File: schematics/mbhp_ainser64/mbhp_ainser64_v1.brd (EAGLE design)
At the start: 100 x 80 mm, 43 parts, among them IC1 MCP3208, IC10 4051, IC11 4051, IC2 74HC595, IC3 7805, IC4 4051, IC5 4051, IC6 4051, IC7 4051, IC8 4051, IC9 4051

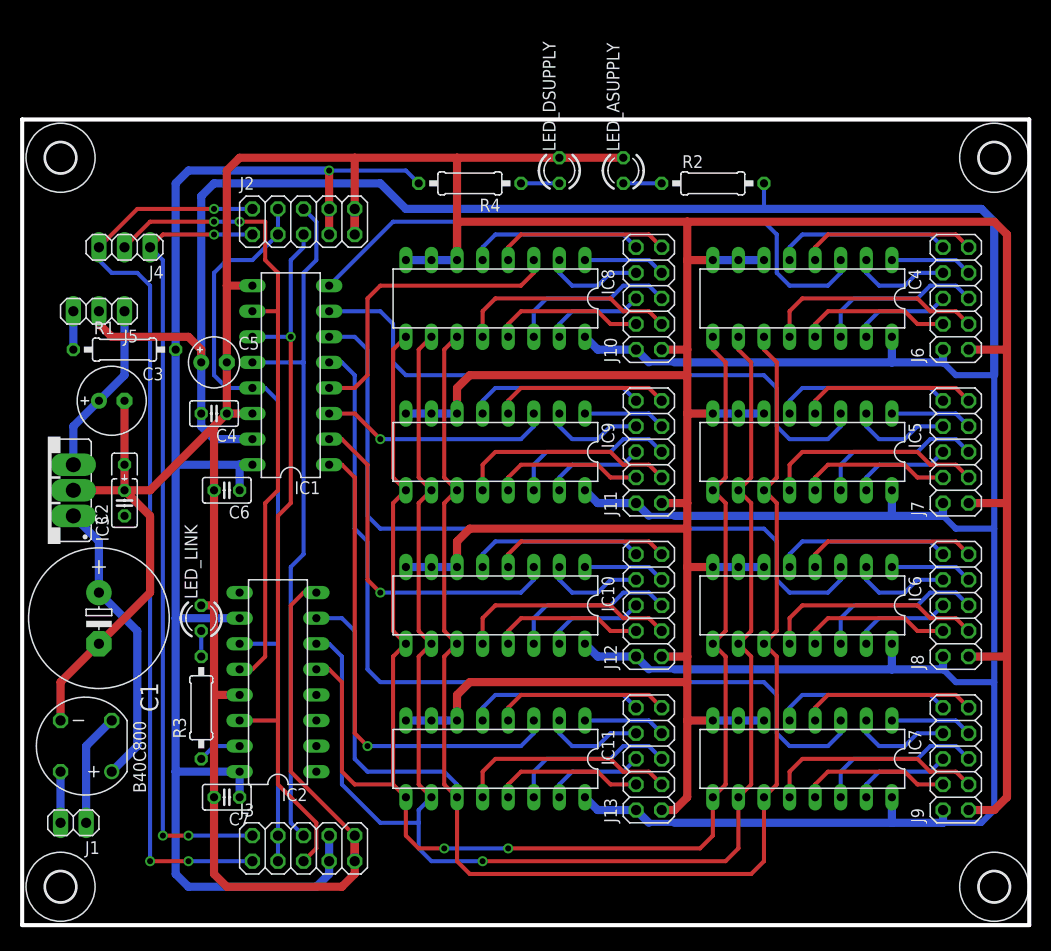
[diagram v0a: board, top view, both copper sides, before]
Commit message: MBHP_AINSER64: layout updates
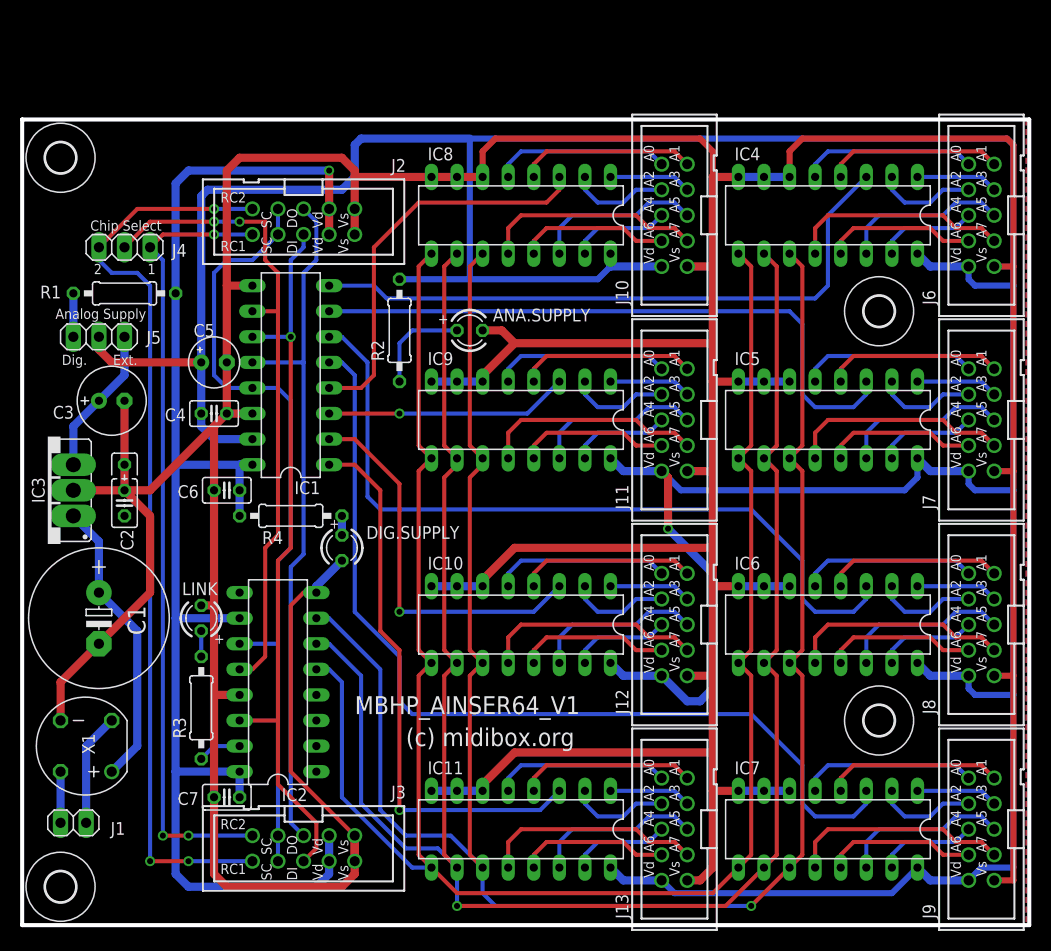
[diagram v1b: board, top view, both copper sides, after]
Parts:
- removed LED_ASUPPLY, LED_DSUPPLY: (no value), led:LED3MM
- added ANA.SUPPLY, DIG.SUPPLY: (no value), led:LED3MM
- J10, J11, J12, J13, J2, J3, J6, J7, J8, J9: device pinhead:2X05 -> con-3m:PAK100/2500-10
- X1: value (none) -> B40C800
- moved R4 37.5 mm to (26.7, 40.6)
- moved R2 34.4 mm to (37.5, 59.1), turned to 90 degrees
- moved E$8 20.1 mm to (85.1, 20.3)
- moved E$7 19.0 mm to (85.1, 61.0)
- moved IC4 8.64 mm to (80.0, 70.5)
- moved J6 8.64 mm to (95.2, 70.5)
- moved IC8 8.64 mm to (49.5, 70.5)
- moved J10 8.64 mm to (64.8, 70.5)
- moved IC7 7.43 mm to (80.0, 9.53)
- moved J9 7.43 mm to (95.2, 9.53)
- moved IC11 7.43 mm to (49.5, 9.53)
- moved J13 7.43 mm to (64.8, 9.53)
- moved R1 5.59 mm to (10.2, 62.7)
- moved IC5 4.07 mm to (80.0, 50.2)
- moved J7 4.07 mm to (95.2, 50.2)
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- renumbered B40C800 to X1, LED_LINK to LINK
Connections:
- net S$70 renamed S$80
- removed net S$10: IC5.5, J7.10
- removed net S$20: IC6.4, J8.9
- removed net S$30: IC7.2, J9.8
- removed net S$40: IC8.1, J10.7
- removed net S$50: IC9.15, J11.6
- removed net S$60: IC10.14, J12.5
- new net S$74: IC11.4, J13.9
- new net S$75: IC11.2, J13.8
- new net S$76: IC11.1, J13.7
- new net S$77: IC11.15, J13.6
- new net S$79: IC11.14, J13.5
- new net S$81: IC11.12, J13.3
- net DI: now also J2.6, J3.6; no longer J2.5, J3.5
- net DO: now also J2.5, J3.5; no longer J2.6, J3.6
- net GND: now also ANA.SUPPLY.K, DIG.SUPPLY.K, J2.1, J2.2, J3.1, J3.2; no longer J2.10, J2.9, J3.10, J3.9, LED_ASUPPLY.K, LED_DSUPPLY.K
- net RC1: now also J2.9, J3.10; no longer J2.2, J3.1
- net RC2: now also J2.10, J3.9; no longer J2.1, J3.2
- net S$11: now also IC5.5, J7.10; no longer IC5.4, J7.9
- net S$12: now also IC5.4, J7.9; no longer IC5.2, J7.8
- net S$13: now also IC5.2, J7.8; no longer IC5.1, J7.7
- net S$14: now also IC5.1, J7.7; no longer IC5.15, J7.6
- net S$15: now also IC5.15, J7.6; no longer IC5.14, J7.5
- net S$16: now also IC5.14, J7.5; no longer IC5.13, J7.4
- net S$17: now also IC5.13, J7.4; no longer IC5.12, J7.3
- net S$19: now also IC5.12, J7.3; no longer IC6.5, J8.10
- net S$21: now also IC6.5, J8.10; no longer IC6.2, J8.8
- net S$22: now also IC6.4, J8.9; no longer IC6.1, J8.7
- net S$23: now also IC6.2, J8.8; no longer IC6.15, J8.6
- net S$24: now also IC6.1, J8.7; no longer IC6.14, J8.5
- net S$25: now also IC6.15, J8.6; no longer IC6.13, J8.4
- net S$26: now also IC6.14, J8.5; no longer IC6.12, J8.3
- net S$28: now also IC6.13, J8.4; no longer IC7.5, J9.10
- net S$29: now also IC6.12, J8.3; no longer IC7.4, J9.9
- net S$31: now also IC7.5, J9.10; no longer IC7.1, J9.7
- net S$32: now also IC7.4, J9.9; no longer IC7.15, J9.6
- net S$33: now also IC7.2, J9.8; no longer IC7.14, J9.5
- net S$34: now also IC7.1, J9.7; no longer IC7.13, J9.4
- net S$35: now also IC7.15, J9.6; no longer IC7.12, J9.3
- net S$37: now also IC7.14, J9.5; no longer IC8.5, J10.10
- net S$38: now also IC7.13, J9.4; no longer IC8.4, J10.9
- net S$39: now also IC7.12, J9.3; no longer IC8.2, J10.8
- net S$41: now also IC8.5, J10.10; no longer IC8.15, J10.6
- net S$42: now also IC8.4, J10.9; no longer IC8.14, J10.5
- net S$43: now also IC8.2, J10.8; no longer IC8.13, J10.4
- net S$44: now also IC8.1, J10.7; no longer IC8.12, J10.3
- net S$46: now also IC8.15, J10.6; no longer IC9.5, J11.10
- net S$47: now also IC8.14, J10.5; no longer IC9.4, J11.9
- net S$48: now also IC8.13, J10.4; no longer IC9.2, J11.8
- net S$49: now also IC8.12, J10.3; no longer IC9.1, J11.7
- net S$51: now also IC9.5, J11.10; no longer IC9.14, J11.5
- net S$52: now also IC9.4, J11.9; no longer IC9.13, J11.4
- net S$53: now also IC9.2, J11.8; no longer IC9.12, J11.3
- net S$55: now also IC9.1, J11.7; no longer IC10.5, J12.10
- net S$56: now also IC9.15, J11.6; no longer IC10.4, J12.9
- net S$57: now also IC9.14, J11.5; no longer IC10.2, J12.8
- net S$58: now also IC9.13, J11.4; no longer IC10.1, J12.7
- net S$59: now also IC9.12, J11.3; no longer IC10.15, J12.6
- net S$61: now also IC10.5, J12.10; no longer IC10.13, J12.4
- net S$62: now also IC10.4, J12.9; no longer IC10.12, J12.3
- net S$64: now also IC10.2, J12.8; no longer IC11.5, J13.10
- net S$65: now also IC10.1, J12.7; no longer IC11.4, J13.9
- net S$66: now also IC10.15, J12.6; no longer IC11.2, J13.8
- net S$67: now also IC10.14, J12.5; no longer IC11.1, J13.7
- net S$68: now also IC10.13, J12.4; no longer IC11.15, J13.6
- net S$69: now also IC10.12, J12.3; no longer IC11.14, J13.5
- net S$71: now also IC11.5, J13.10; no longer IC11.12, J13.3
- net S$72: now also ANA.SUPPLY.A; no longer LED_ASUPPLY.A
- net S$73: now also DIG.SUPPLY.A; no longer LED_DSUPPLY.A
- net SC: now also J2.7, J2.8, J3.7, J3.8; no longer J2.3, J2.4, J3.3, J3.4
- net VCC: now also J2.3, J2.4, J3.3, J3.4; no longer J2.7, J2.8, J3.7, J3.8
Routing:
- net MUXA: track 154.5 -> 187.1 mm, vias 2 -> 0
- net MUXB: track 166.2 -> 194.7 mm
- net MUXC: track 171.5 -> 198.3 mm, vias 0 -> 1
- net VCA: track 368.1 -> 393.6 mm, vias 0 -> 1
- net S$81: track 0.00 -> 21.9 mm
- net S$74: track 0.00 -> 17.6 mm
- net S$20: track 17.6 -> 0.00 mm
- net S$10: track 17.6 -> 0.00 mm
- net S$60: track 16.8 -> 0.00 mm
- net S$79: track 0.00 -> 16.8 mm
- net S$49: track 8.15 -> 21.9 mm
- net S$44: track 21.9 -> 8.15 mm
- net S$59: track 9.94 -> 21.9 mm
- net S$53: track 21.9 -> 9.94 mm
- net S$39: track 9.94 -> 21.9 mm
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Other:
- board text added: "(c) midibox.org"
- board text added: "+"
- board text added: "1"
- board text added: "2"
- board text added: "A0"
- board text added: "A1"
- board text added: "A2"
- board text added: "A3"
- board text added: "A4"
- board text added: "A5"
- board text added: "A6"
- board text added: "A7"
- board text added: "Analog Supply"
- board text added: "Chip Select"
- board text added: "DI"
- board text added: "DO"
- board text added: "Dig."
- board text added: "Ext."
- board text added: "MBHP_AINSER64_V1"
- board text added: "RC1"
- board text added: "RC2"
- board text added: "SC"
- board text added: "Vd"
- board text added: "Vs"
